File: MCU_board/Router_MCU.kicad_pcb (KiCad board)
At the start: 2 copper layers, 157.6 x 116.2 mm, 72 parts, among them J1 Header, T1 HY601742, U1 MYC-YT507H, U2 TPS54540, U3 LAN8720A, X1 S4B-XH, X2 S4B-XH, X3 S4B-XH, X4 S4B-XH, X5 B2B-XH, X6 TFP09-2-12B, X7 RJ45, Y1 25MHz

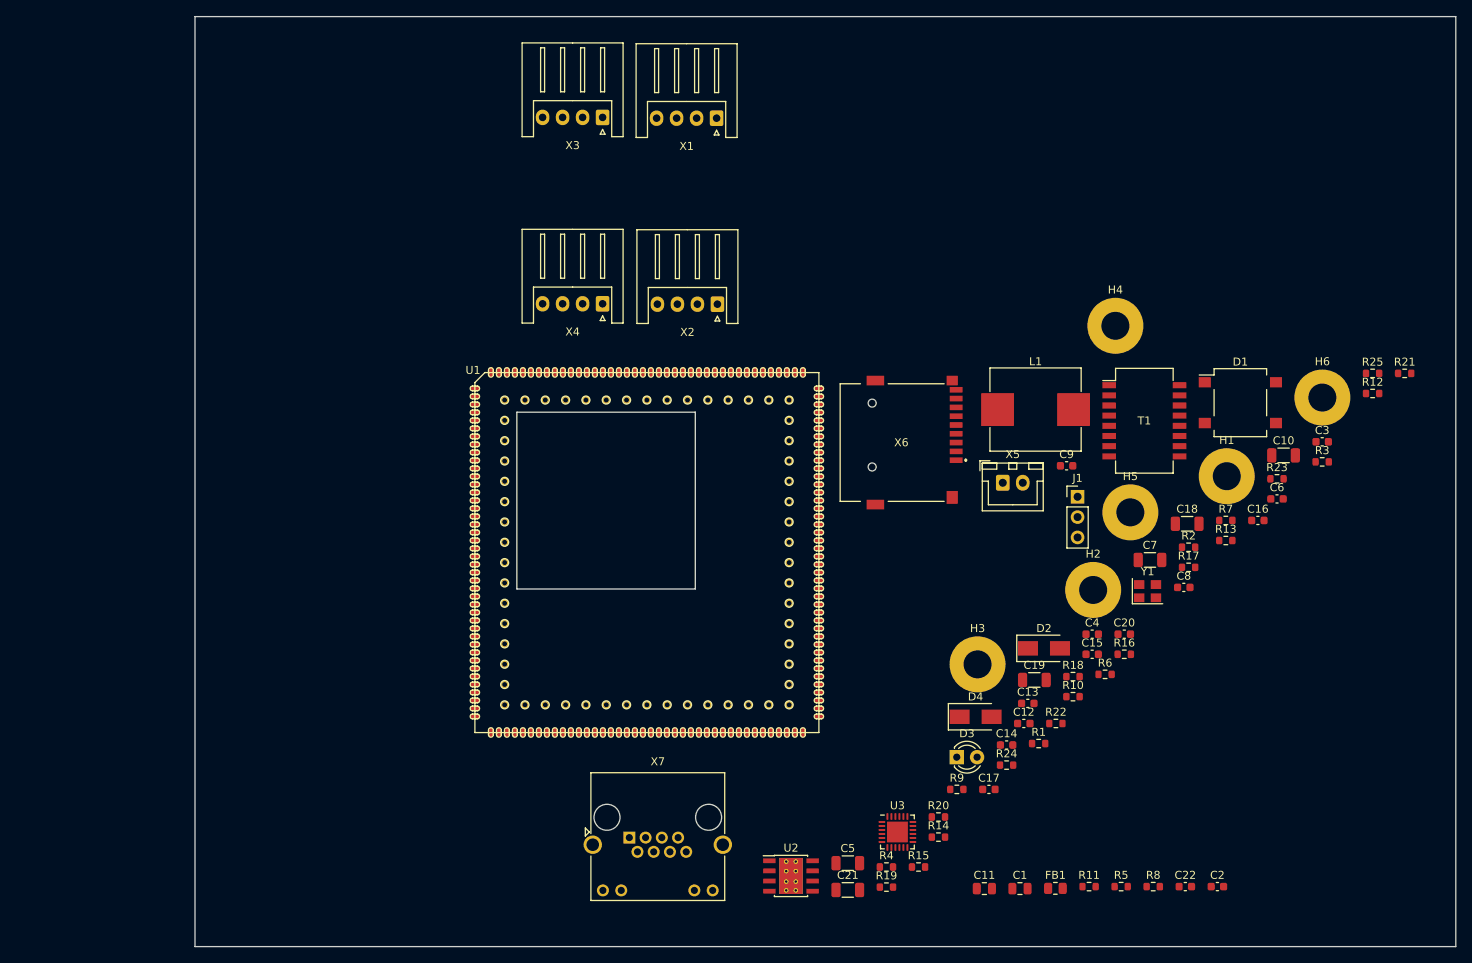
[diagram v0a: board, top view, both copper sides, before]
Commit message: routing procs
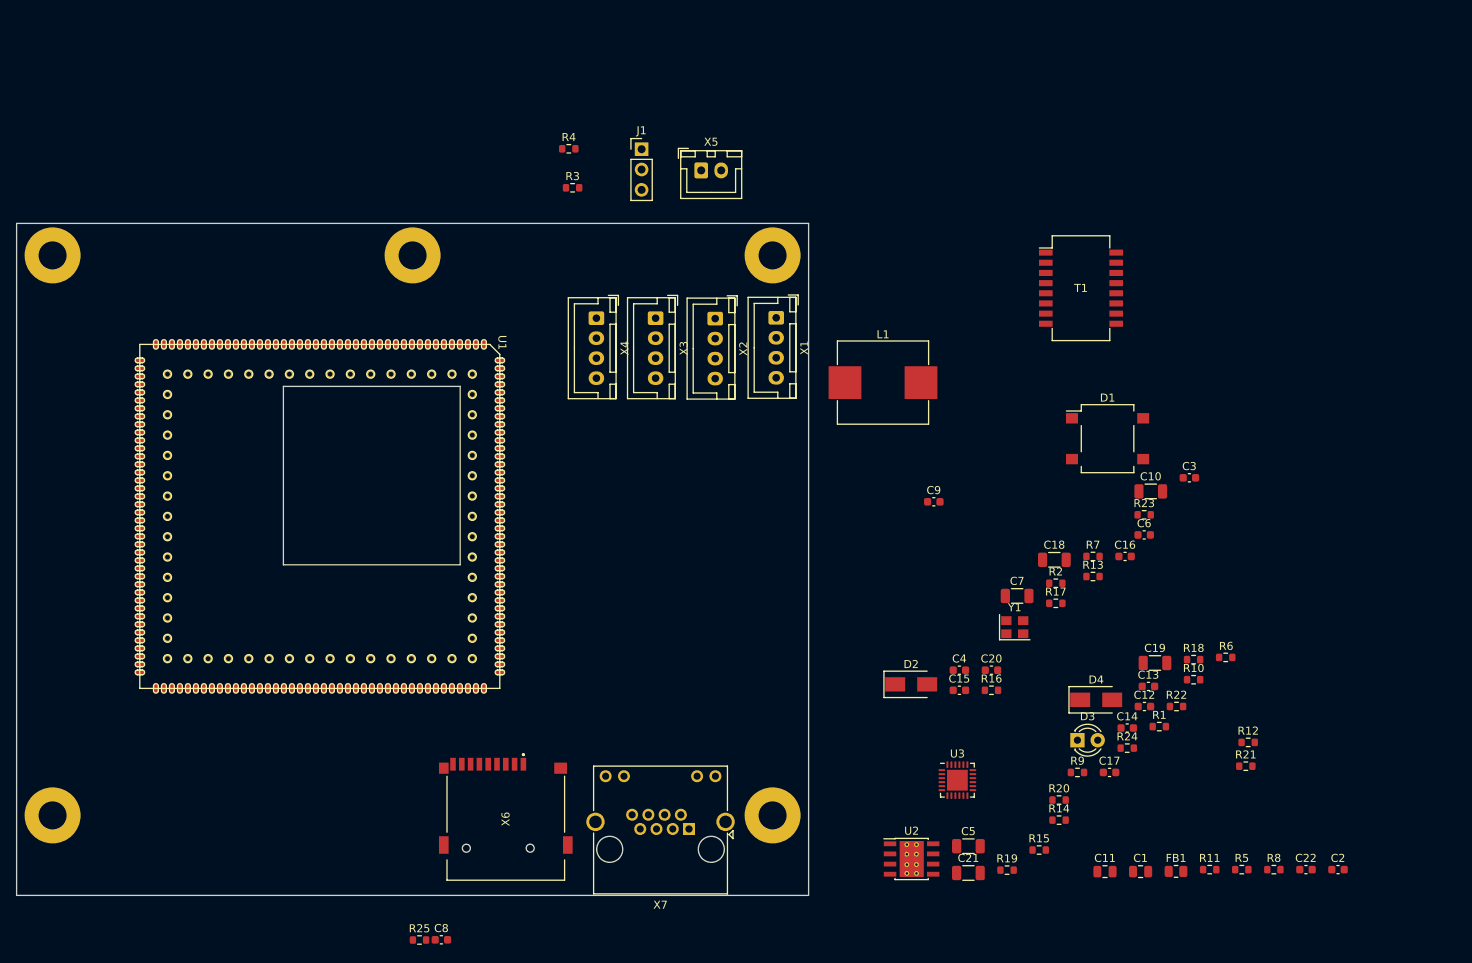
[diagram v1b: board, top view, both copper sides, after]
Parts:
- removed H6: M3, MountingHole:MountingHole_3.5mm_Pad
- X1, X2, X3, X4: value S4B-XH -> B4B-XH; footprint Connector_JST:JST_XH_S4B-XH-A_1x04_P2.50mm_Horizontal -> Connector_JST:JST_XH_B4B-XH-A_1x04_P2.50mm_Vertical
- moved H1 149.3 mm to (116.3, 76.8)
- moved R25 138.6 mm to (162.2, 162.4)
- moved H3 117.2 mm to (116.3, 146.8)
- moved C8 102.7 mm to (164.9, 162.4)
- moved R3 99.8 mm to (181.3, 68.4)
- moved R4 98.2 mm to (180.9, 63.5)
- moved H5 95.3 mm to (161.3, 76.8)
- moved H4 74.7 mm to (206.3, 146.8)
- moved J1 69.7 mm to (190.0, 63.6)
- moved X6 68.8 mm to (173.0, 154.9), turned to 90 degrees
- moved H2 57.9 mm to (206.3, 76.8)
- moved X5 54.3 mm to (197.4, 66.2)
- moved R21 53.0 mm to (265.5, 140.7)
- moved R12 46.3 mm to (265.8, 137.7)
- moved U1 44.5 mm to (147.8, 110.9), turned to -90 degrees
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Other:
- board size 157.6 x 116.2 mm -> 99 x 84 mm
